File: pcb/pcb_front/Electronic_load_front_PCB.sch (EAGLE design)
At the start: 12 parts, among them SW1 EC12E_SW

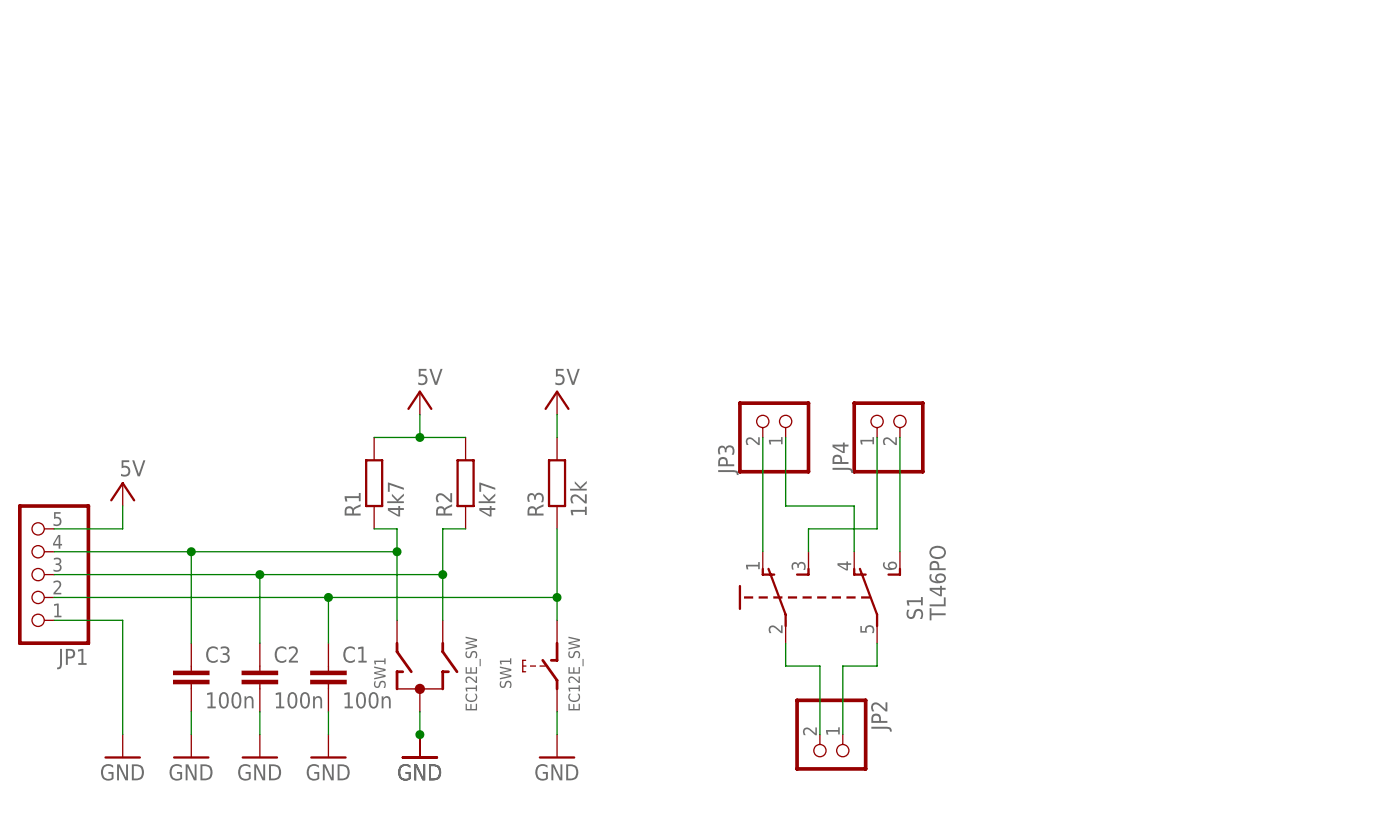
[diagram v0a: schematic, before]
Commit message: cleanup
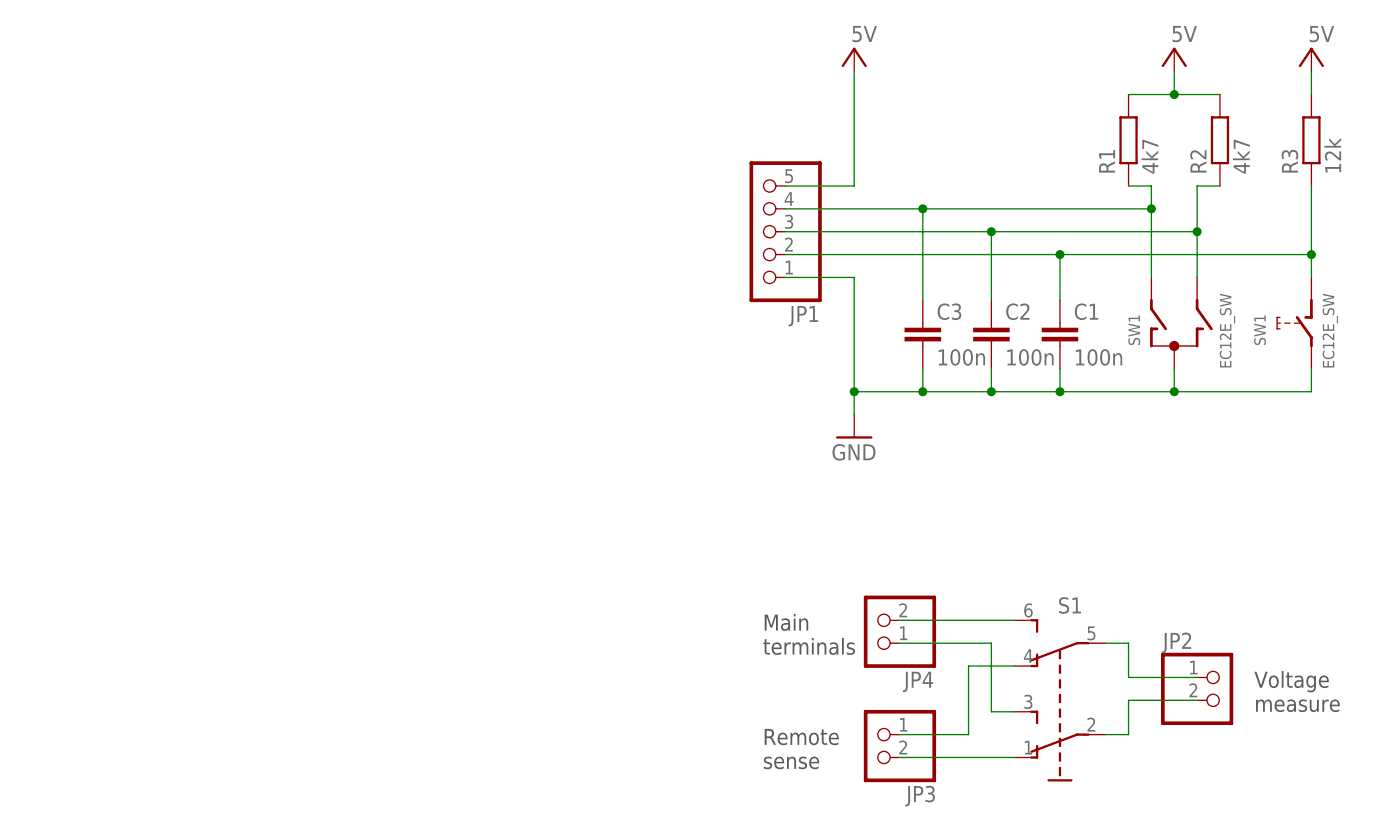
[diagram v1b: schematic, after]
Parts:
- JP1: device pinhead:PINHD-1X5/90 -> pinhead:PINHD-1X5
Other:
- note added: "Main terminals"
- note added: "Remote sense"
- note added: "Rotary encoder"
- note added: "V measurement source selector"
- note added: "Voltage measure"
- moved on the sheet: C1, C2, C3, JP1, JP2, JP3, JP4, R1, R2, R3, S1, SW1
